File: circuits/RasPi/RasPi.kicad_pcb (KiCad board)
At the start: 2 copper layers, 90 x 57 mm, 276 parts, among them J1 Conn_01x14_Pin, J12 Conn_01x02_MountingPin, J13 Conn_01x03_MountingPin, J14 Conn_01x02_MountingPin, J15 USB_C_Receptacle_USB2.0, J2 Conn_01x06_MountingPin, J3 Conn_01x06_MountingPin, J5 Conn_01x05_Pin, J6 Conn_01x03_MountingPin, J7 RJ45_Hanrun_HR911105A_Horizon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, J8 Conn_01x07_MountingPin, J9 Conn_01x04_MountingPin, Q1 S8550, Q10 BSS138, Q12 SSM6J808R, Q13 BSS138, Q14 SSM6J808R, Q15 S8550, Q16 SSM3J332R, Q17 S8550, Q18 S8550, Q19 S8550, Q2 S8550, Q20 BSS138, Q21 BSS138, Q22 S8550, Q23 BSS138, Q25 BSS138, Q26 SSM3J332R, Q27 BSS138, Q28 SSM3J332R, Q29 BSS138, Q3 S8550, Q30 BSS138, Q33 BSS138, Q4 S8550, Q5 S8550, Q6 SSM3J332R, Q7 S8550, Q8 SSM3J332R, Q9 S8550, SW1 SW_SPST, SW2 SW_DIP_x04, SW3 SW_SPDT, SW4 SW_SPDT_White, SW5 SW_SPDT, SW6 SW_SPDT, SW7 SW_SPST, U1 STM32F446RETx, U10 MAX3485, U11 MAX3485, U12 MAX3485, U13 TPS54560BDDA, U14 MAX3485, U15 STM32H723VGTx, U16 AZ1117CH-3.3, U17 M51957B, U18 DAC_PT8211S, U19 DCDC_TPS61023, U2 MAX3485, U20 FT231XS, U3 MAX3485, U4 MAX3485, U5 MAX3485, U6 SBC_RPi-CM4, U7 FPGA_TangPrimer25K_Core, U8 MAX3485, U9 MAX3485, Y1 16MHz

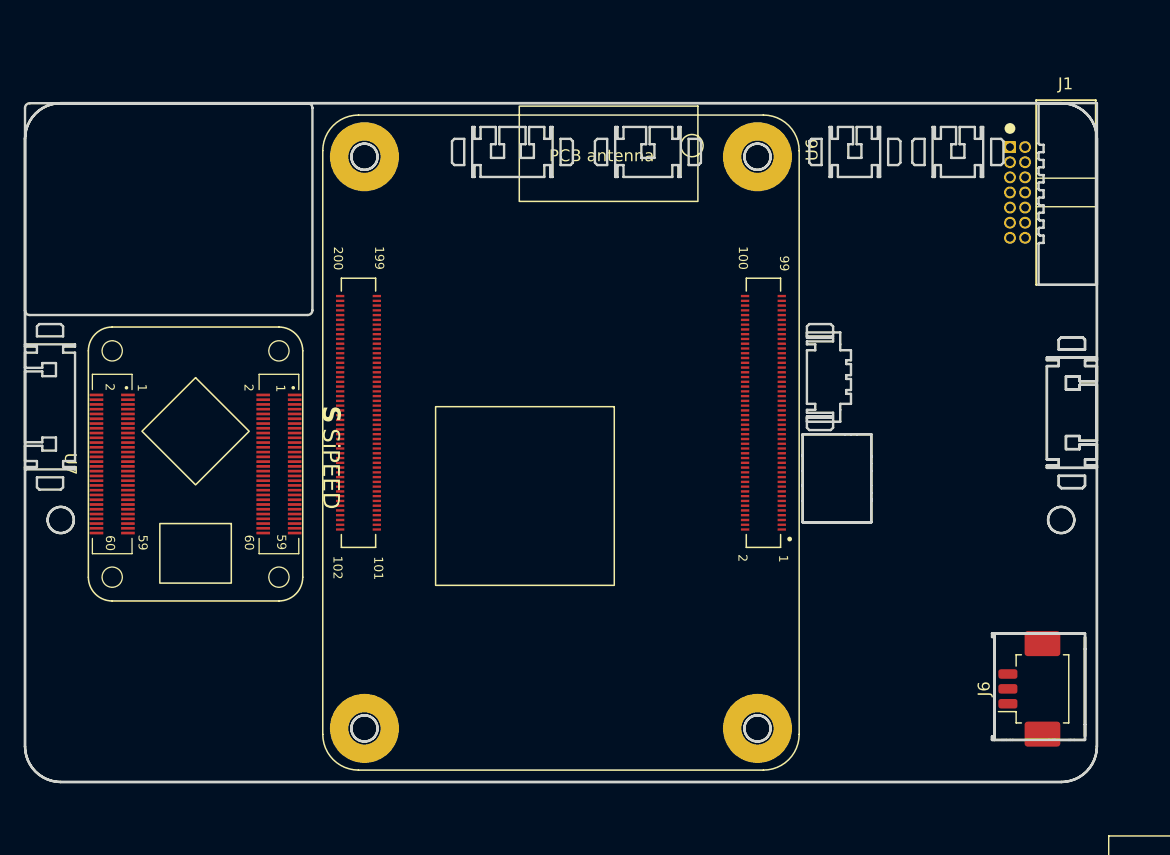
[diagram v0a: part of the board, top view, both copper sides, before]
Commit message: 配線
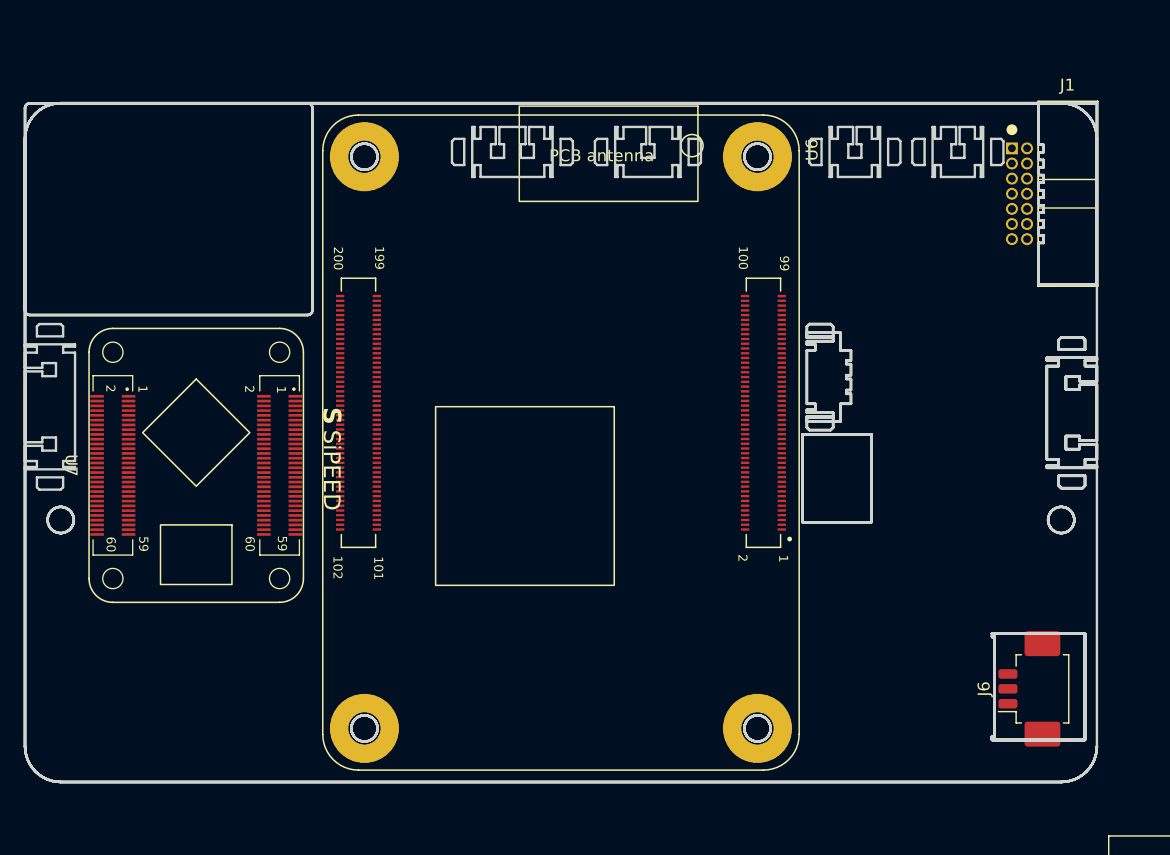
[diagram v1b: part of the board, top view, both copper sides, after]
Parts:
- moved J1 0.20 mm to (37.9, -20.9)
- moved U7 0.13 mm to (-30.6, 1.92)
